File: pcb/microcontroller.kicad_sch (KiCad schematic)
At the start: 24 parts, among them J1 TC2030, J3 TC2030, U3 74HCT541, U4 STM32F103C8T6, U5 SN65HVD230, Y1 8MHz

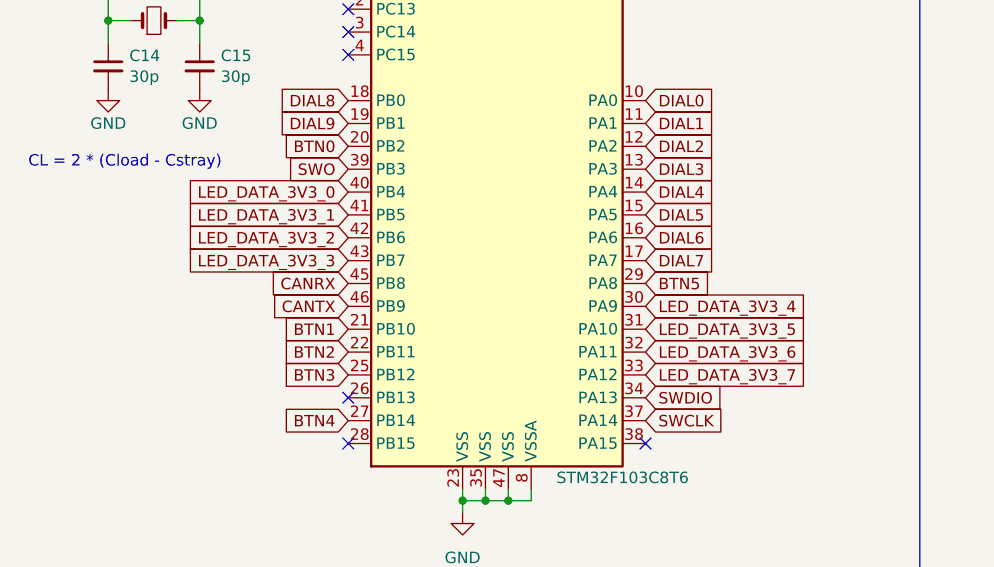
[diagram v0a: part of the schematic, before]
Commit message: PCB layout work
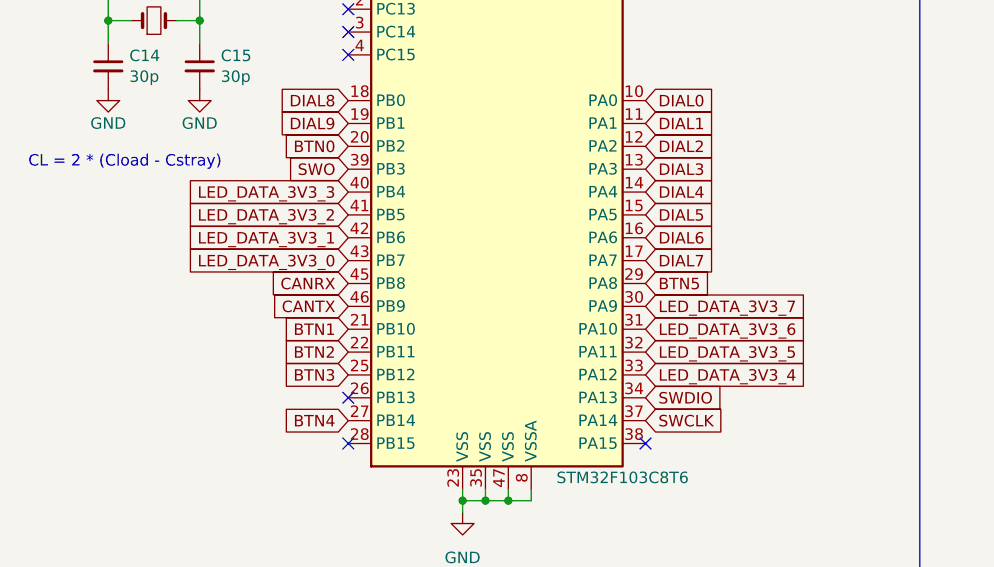
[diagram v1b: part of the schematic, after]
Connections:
- net LED_DATA_3V3_0: now also U4.43 (PB7); no longer U4.40 (PB4)
- net LED_DATA_3V3_1: now also U4.42 (PB6); no longer U4.41 (PB5)
- net LED_DATA_3V3_2: now also U4.41 (PB5); no longer U4.42 (PB6)
- net LED_DATA_3V3_3: now also U4.40 (PB4); no longer U4.43 (PB7)
- net LED_DATA_3V3_4: now also U4.33 (PA12); no longer U4.30 (PA9)
- net LED_DATA_3V3_5: now also U4.32 (PA11); no longer U4.31 (PA10)
- net LED_DATA_3V3_6: now also U4.31 (PA10); no longer U4.32 (PA11)
- net LED_DATA_3V3_7: now also U4.30 (PA9); no longer U4.33 (PA12)
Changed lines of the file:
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@@
     )
   )
-  (global_label "LED_DATA_3V3_7" (shape input) (at 104.14 130.81 0) (fields_autoplaced)
-    (effects (font (size 1.27 1.27)) (justify left))
-    (property "Intersheet References" "${INTERSHEET_REFS}" (id 0) (at 122.035 130.7306 0)
+  (global_label "LED_DATA_3V3_7" (shape input) (at 104.14 123.19 0) (fields_autoplaced)
+    (effects (font (size 1.27 1.27)) (justify left))
+    (property "Intersheet References" "${INTERSHEET_REFS}" (id 0) (at 122.035 123.2694 0)
       (effects (font (size 1.27 1.27)) (justify left) hide)
     )
@@
     )
   )
-  (global_label "LED_DATA_3V3_3" (shape input) (at 71.12 118.11 180) (fields_autoplaced)
-    (effects (font (size 1.27 1.27)) (justify right))
-    (property "Intersheet References" "${INTERSHEET_REFS}" (id 0) (at 53.225 118.0306 0)
+  (global_label "LED_DATA_3V3_3" (shape input) (at 71.12 110.49 180) (fields_autoplaced)
+    (effects (font (size 1.27 1.27)) (justify right))
+    (property "Intersheet References" "${INTERSHEET_REFS}" (id 0) (at 53.225 110.5694 0)
       (effects (font (size 1.27 1.27)) (justify right) hide)
     )
@@
     )
   )
-  (global_label "LED_DATA_3V3_0" (shape input) (at 71.12 110.49 180) (fields_autoplaced)
-    (effects (font (size 1.27 1.27)) (justify right))
-    (property "Intersheet References" "${INTERSHEET_REFS}" (id 0) (at 53.225 110.4106 0)
+  (global_label "LED_DATA_3V3_0" (shape input) (at 71.12 118.11 180) (fields_autoplaced)
+    (effects (font (size 1.27 1.27)) (justify right))
+    (property "Intersheet References" "${INTERSHEET_REFS}" (id 0) (at 53.225 118.1894 0)
       (effects (font (size 1.27 1.27)) (justify right) hide)
     )
@@
     )
   )
-  (global_label "LED_DATA_3V3_5" (shape input) (at 104.14 125.73 0) (fields_autoplaced)
-    (effects (font (size 1.27 1.27)) (justify left))
-    (property "Intersheet References" "${INTERSHEET_REFS}" (id 0) (at 122.035 125.6506 0)
+  (global_label "LED_DATA_3V3_5" (shape input) (at 104.14 128.27 0) (fields_autoplaced)
+    (effects (font (size 1.27 1.27)) (justify left))
+    (property "Intersheet References" "${INTERSHEET_REFS}" (id 0) (at 122.035 128.3494 0)
       (effects (font (size 1.27 1.27)) (justify left) hide)
     )
@@
     )
   )
-  (global_label "LED_DATA_3V3_6" (shape input) (at 104.14 128.27 0) (fields_autoplaced)
-    (effects (font (size 1.27 1.27)) (justify left))
-    (property "Intersheet References" "${INTERSHEET_REFS}" (id 0) (at 122.035 128.1906 0)
+  (global_label "LED_DATA_3V3_6" (shape input) (at 104.14 125.73 0) (fields_autoplaced)
+    (effects (font (size 1.27 1.27)) (justify left))
+    (property "Intersheet References" "${INTERSHEET_REFS}" (id 0) (at 122.035 125.8094 0)
       (effects (font (size 1.27 1.27)) (justify left) hide)
     )
@@
     )
   )
-  (global_label "LED_DATA_3V3_1" (shape input) (at 71.12 113.03 180) (fields_autoplaced)
-    (effects (font (size 1.27 1.27)) (justify right))
-    (property "Intersheet References" "${INTERSHEET_REFS}" (id 0) (at 53.225 112.9506 0)
-      (effects (font (size 1.27 1.27)) (justify right) hide)
-    )
-  )
-  (global_label "LED_DATA_3V3_4" (shape input) (at 104.14 123.19 0) (fields_autoplaced)
-    (effects (font (size 1.27 1.27)) (justify left))
-    (property "Intersheet References" "${INTERSHEET_REFS}" (id 0) (at 122.035 123.1106 0)
+  (global_label "LED_DATA_3V3_1" (shape input) (at 71.12 115.57 180) (fields_autoplaced)
+    (effects (font (size 1.27 1.27)) (justify right))
+    (property "Intersheet References" "${INTERSHEET_REFS}" (id 0) (at 53.225 115.6494 0)
+      (effects (font (size 1.27 1.27)) (justify right) hide)
+    )
+  )
+  (global_label "LED_DATA_3V3_4" (shape input) (at 104.14 130.81 0) (fields_autoplaced)
+    (effects (font (size 1.27 1.27)) (justify left))
+    (property "Intersheet References" "${INTERSHEET_REFS}" (id 0) (at 122.035 130.8894 0)
       (effects (font (size 1.27 1.27)) (justify left) hide)
     )
@@
     )
   )
-  (global_label "LED_DATA_3V3_2" (shape input) (at 71.12 115.57 180) (fields_autoplaced)
-    (effects (font (size 1.27 1.27)) (justify right))
-    (property "Intersheet References" "${INTERSHEET_REFS}" (id 0) (at 53.225 115.4906 0)
-      (effects (font (size 1.27 1.27)) (justify right) hide)
-    )
+  (global_label "LED_DATA_3V3_2" (shape input) (at 71.12 113.03 180) (fields_autoplaced)
+    (effects (font (size 1.27 1.27)) (justify right))
+    (property "Intersheet References" "${INTERSHEET_REFS}" (id 0) (at 53.225 113.1094 0)
+      (effects (font (size 1.27 1.27)) (justify right) hide)
+    )
